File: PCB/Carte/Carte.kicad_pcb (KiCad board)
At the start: 2 copper layers, 99 x 83.8 mm, 13 parts, among them J1 Conn_01x02_Pin, J2 Conn_01x02_Pin, J3 Conn_01x02_Pin, J4 Conn_01x02_Pin, J5 Conn_01x02_Pin, J6 Conn_01x01_Pin, J7 Conn_01x01_Pin, J8 1Pin

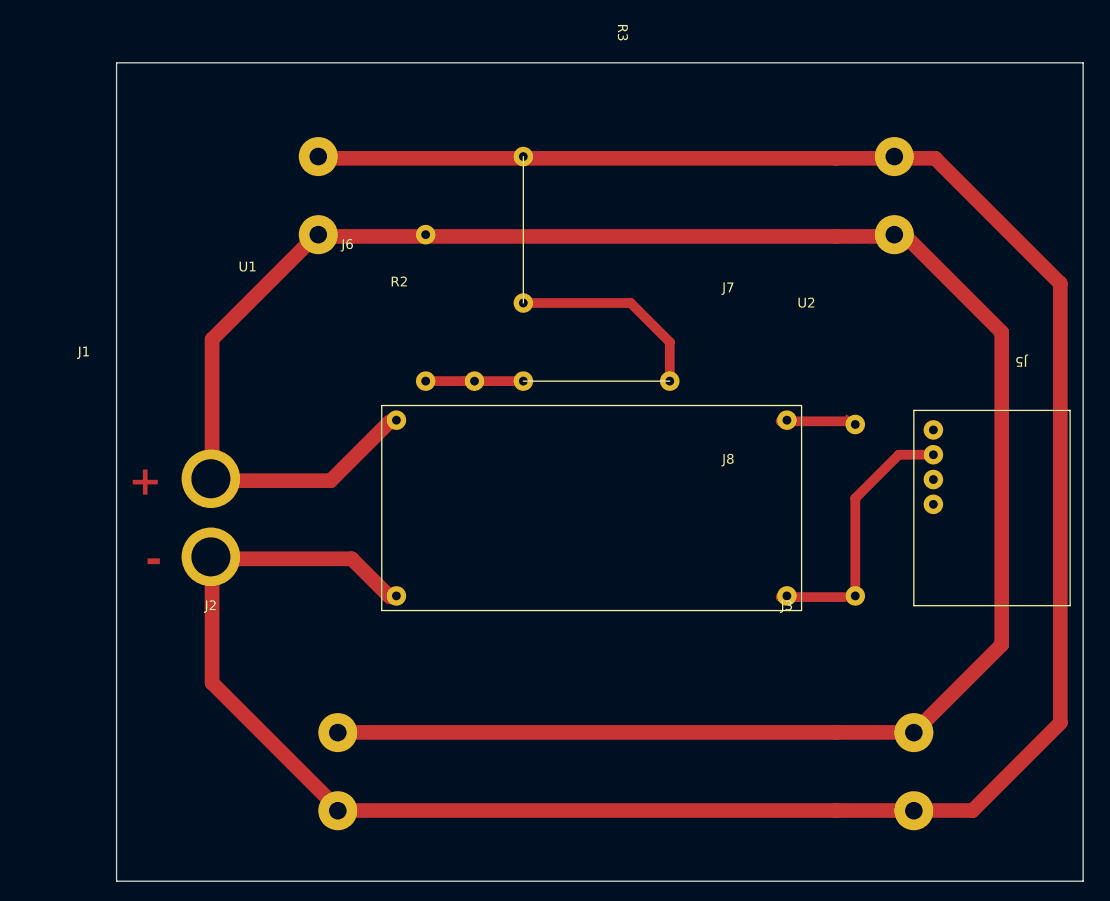
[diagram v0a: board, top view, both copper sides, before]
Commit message: PCB
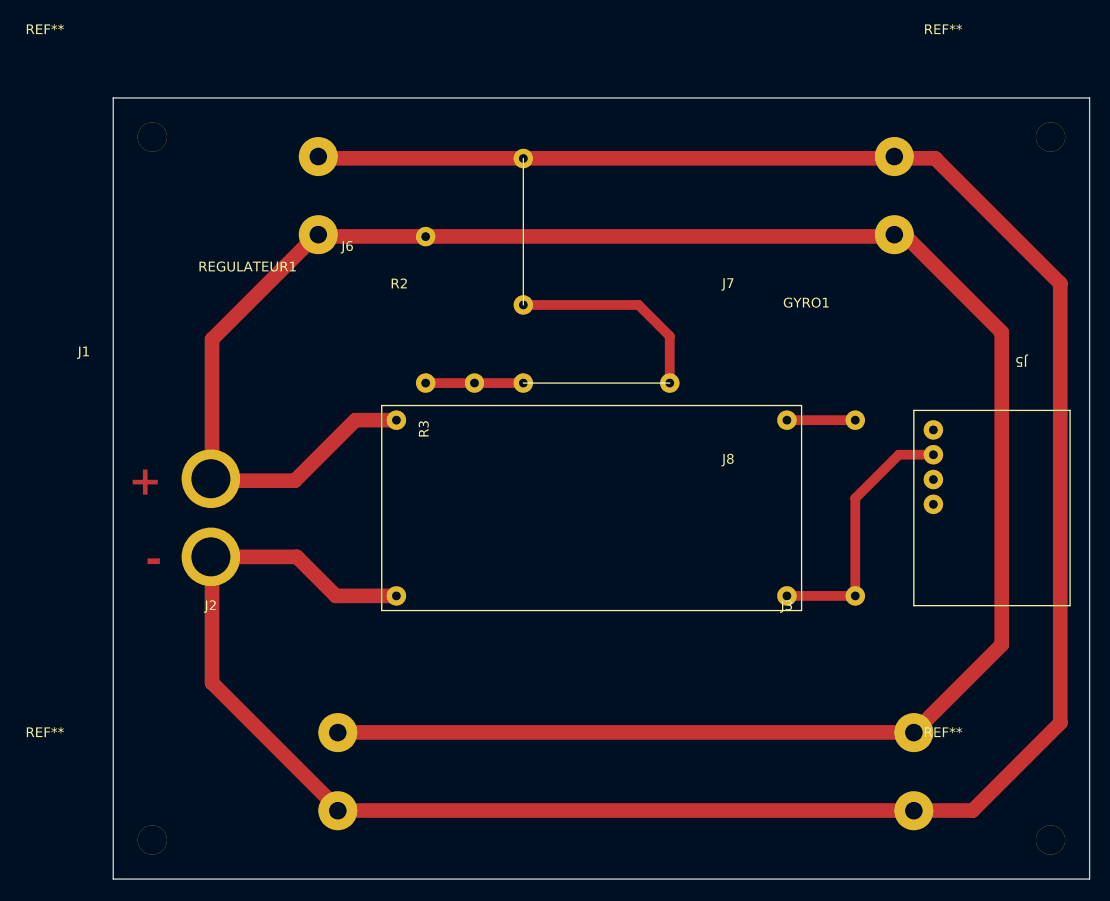
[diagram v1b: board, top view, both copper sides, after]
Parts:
- added REF**: Trou, my_lib:Trou, F.Cu at (57.0, 105.0)
- added REF**: Trou, my_lib:Trou, F.Cu at (57.0, 33.0)
- added REF**: Trou, my_lib:Trou, F.Cu at (149.0, 33.0)
- added REF**: Trou, my_lib:Trou, F.Cu at (149.0, 105.0)
- J1: value Conn_01x02_Pin -> LIPO
- J2, J3, J4, J5: value Conn_01x02_Pin -> ESC
- J6: value Conn_01x01_Pin -> to GPIO
- J7: value Conn_01x01_Pin -> to 5V
- J8: value 1Pin -> to GND
- moved R3 15.2 mm to (95.0, 50.2), turned to 90 degrees
- moved R1 14.8 mm to (85.0, 43.2), turned to -90 degrees
- moved J7 0.44 mm to (129.0, 62.0)
- moved J6 0.20 mm to (90.0, 58.2)
- moved R2 0.20 mm to (95.0, 58.2)
- renumbered U2 to GYRO1, U1 to REGULATEUR1
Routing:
- net Net-(GYRO1-GND): track 18.8 -> 25.8 mm
- net Net-(J1-Pin_2): track 262.0 -> 256.0 mm
- net Net-(J1-Pin_1): track 228.6 -> 229.3 mm
- net Net-(J7-Pin_1): track 7.77 -> 7.08 mm
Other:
- board size 99 x 83.8 mm -> 100 x 80 mm
